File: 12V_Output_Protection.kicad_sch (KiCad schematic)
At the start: 6 parts, among them U16 VND7050AJTR

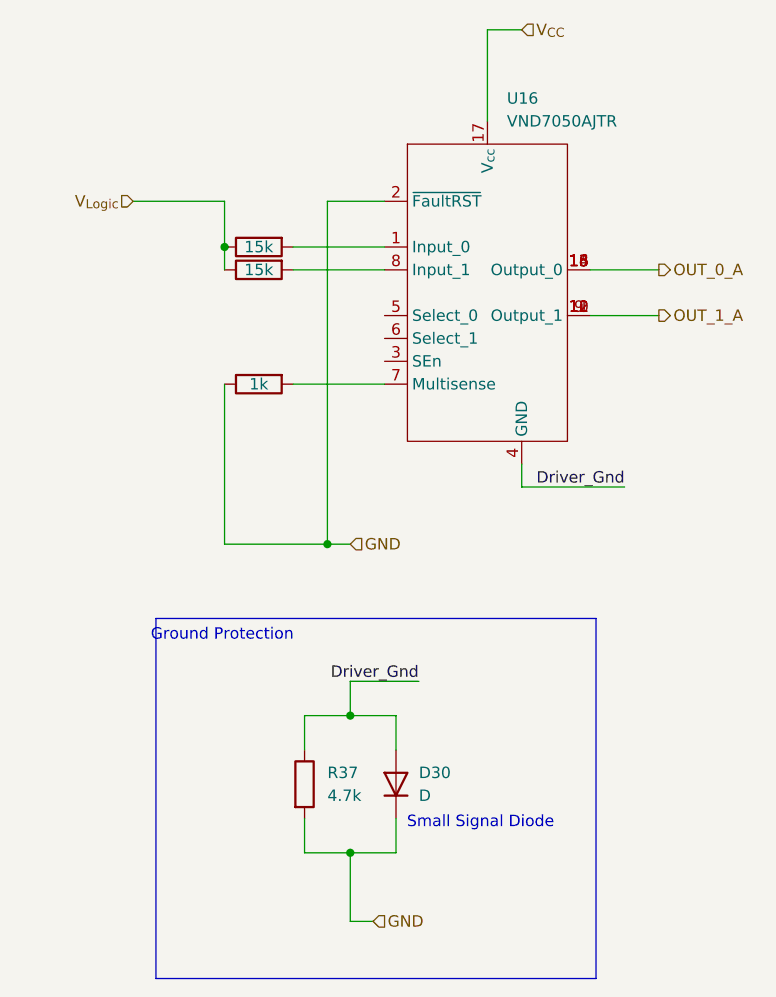
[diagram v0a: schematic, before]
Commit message: All the diodes, and other layout work
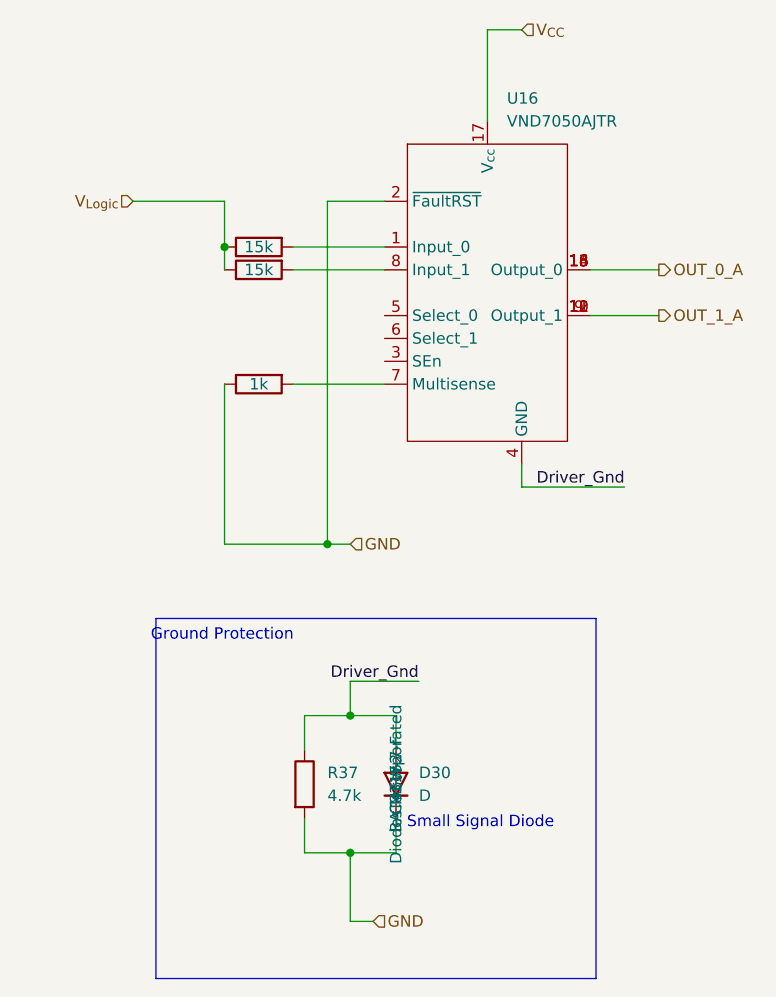
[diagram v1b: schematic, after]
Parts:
- D30: footprint Diode_SMD:D_0805_2012Metric -> Diode_SMD:D_SOD-123; LCSC (none) -> C83152; MPN (none) -> BAT46W-7-F; Manufacturer (none) -> Diodes Incorporated
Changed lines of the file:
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@@
 			)
 		)
-		(property "Footprint" "Diode_SMD:D_0805_2012Metric"
+		(property "Footprint" "Diode_SMD:D_SOD-123"
 			(at 130.81 148.59 0)
 			(effects
@@
 			)
 		)
-		(property "Datasheet" "~"
+		(property "Datasheet" "https://www.lcsc.com/datasheet/lcsc_datasheet_2412251151_Diodes-Incorporated-BAT46W-7-F_C83152.pdf"
 			(at 130.81 148.59 0)
 			(effects
@@
 			)
 		)
+		(property "LCSC" "C83152"
+			(at 130.81 148.59 0)
+			(effects
+				(font
+					(size 1.27 1.27)
+				)
+			)
+		)
+		(property "MPN" "BAT46W-7-F"
+			(at 130.81 148.59 0)
+			(effects
+				(font
+					(size 1.27 1.27)
+				)
+			)
+		)
+		(property "Manufacturer" "Diodes Incorporated"
+			(at 130.81 148.59 0)
+			(effects
+				(font
+					(size 1.27 1.27)
+				)
+			)
+		)
